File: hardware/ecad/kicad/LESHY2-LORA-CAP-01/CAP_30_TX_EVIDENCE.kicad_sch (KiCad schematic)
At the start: 0 parts

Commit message: complete H2.4.2 LoRa Cap root
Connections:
- no-connect marks 0 -> 4
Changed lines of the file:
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@@
 	(generator_version "10.0")
 	(paper "A4")
+	(hierarchical_label "CAP_3V3"
+		(shape bidirectional)
+		(at 20.32 20.32 0)
+		(effects (font (size 1.27 1.27)))
+	)
+	(wire
+		(pts (xy 20.32 20.32) (xy 25.40 20.32))
+		(stroke (width 0) (type default))
+	)
+	(no_connect (at 25.40 20.32)
+	)
+	(hierarchical_label "GND"
+		(shape bidirectional)
+		(at 20.32 25.40 0)
+		(effects (font (size 1.27 1.27)))
+	)
+	(wire
+		(pts (xy 20.32 25.40) (xy 25.40 25.40))
+		(stroke (width 0) (type default))
+	)
+	(no_connect (at 25.40 25.40)
+	)
+	(hierarchical_label "RF_FORWARD_LEVEL"
+		(shape bidirectional)
+		(at 190.50 20.32 180)
+		(effects (font (size 1.27 1.27)) (justify right))
+	)
+	(wire
+		(pts (xy 190.50 20.32) (xy 185.42 20.32))
+		(stroke (width 0) (type default))
+	)
+	(no_connect (at 185.42 20.32)
+	)
+	(hierarchical_label "EXT_TX_EVIDENCE_N"
+		(shape bidirectional)
+		(at 190.50 25.40 180)
+		(effects (font (size 1.27 1.27)) (justify right))
+	)
+	(wire
+		(pts (xy 190.50 25.40) (xy 185.42 25.40))
+		(stroke (width 0) (type default))
+	)
+	(no_connect (at 185.42 25.40)
+	)
 	(sheet_instances
 		(path "/"

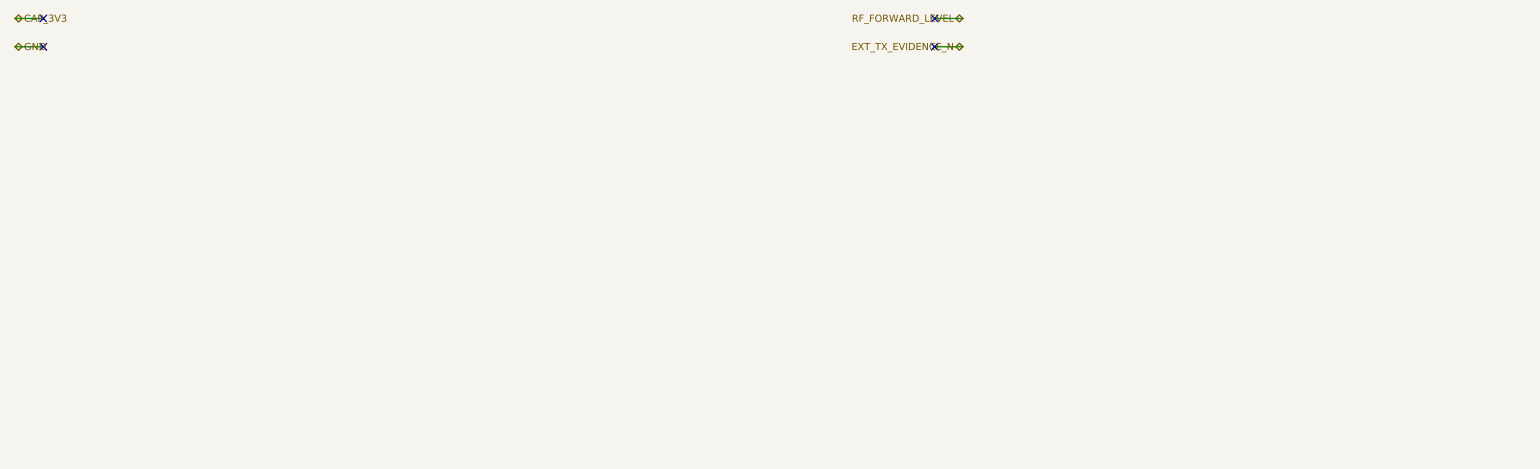
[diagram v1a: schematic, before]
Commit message: complete H2.4 LoRa Cap schematics
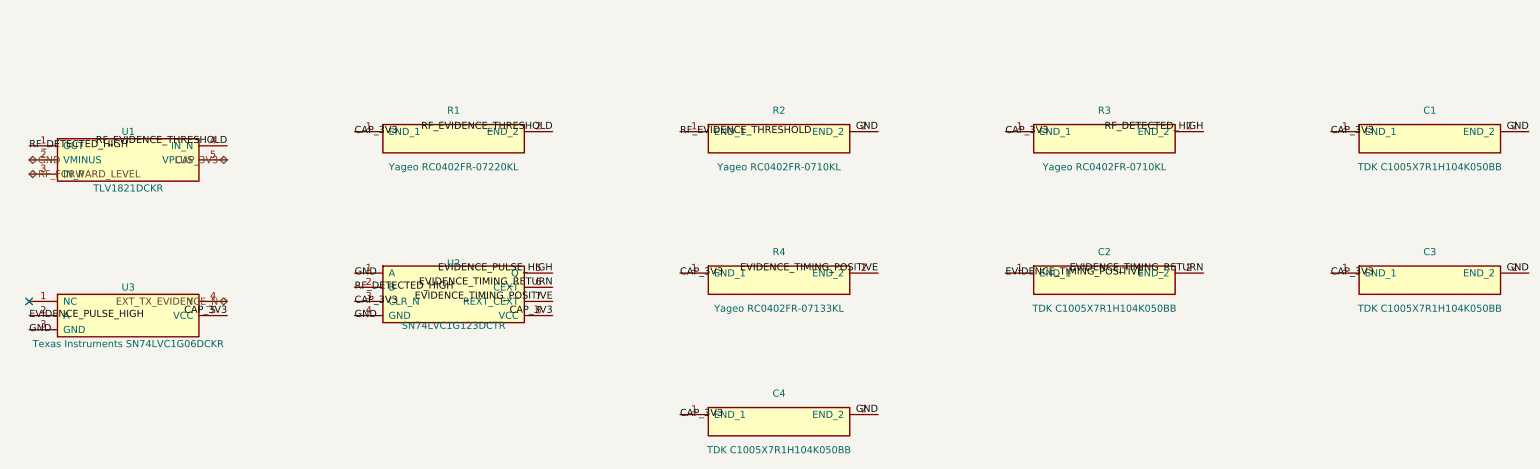
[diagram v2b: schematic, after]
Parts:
- added C1: TDK C1005X7R1H104K050BB, Capacitor_SMD:C_0402_1005Metric, symbol Leshy2:CAP30_EVIDENCE_COMPARATOR_BYPASS
- added C2: TDK C1005X7R1H104K050BB, Capacitor_SMD:C_0402_1005Metric, symbol Leshy2:CAP30_EVIDENCE_TIMING_CAPACITOR
- added C3: TDK C1005X7R1H104K050BB, Capacitor_SMD:C_0402_1005Metric, symbol Leshy2:CAP30_EVIDENCE_MONOSTABLE_BYPASS
- added C4: TDK C1005X7R1H104K050BB, Capacitor_SMD:C_0402_1005Metric, symbol Leshy2:CAP30_EVIDENCE_DRIVER_BYPASS
- added R1: Yageo RC0402FR-07220KL, Resistor_SMD:R_0402_1005Metric, symbol Leshy2:CAP30_EVIDENCE_THRESHOLD_TOP
- added R2: Yageo RC0402FR-0710KL, Resistor_SMD:R_0402_1005Metric, symbol Leshy2:CAP30_EVIDENCE_THRESHOLD_BOTTOM
- added R3: Yageo RC0402FR-0710KL, Resistor_SMD:R_0402_1005Metric, symbol Leshy2:CAP30_EVIDENCE_COMPARATOR_PULLUP
- added R4: Yageo RC0402FR-07133KL, Resistor_SMD:R_0402_1005Metric, symbol Leshy2:CAP30_EVIDENCE_TIMING_RESISTOR
- added U1: TLV1821DCKR, Package_TO_SOT_SMD:Texas_R-PDSO-G5_DCK-5, symbol Leshy2:CAP30_EVIDENCE_COMPARATOR
- added U2: SN74LVC1G123DCTR, Package_SO:SSOP-8_2.95x2.8mm_P0.65mm, symbol Leshy2:CAP30_EVIDENCE_MONOSTABLE
- added U3: Texas Instruments SN74LVC1G06DCKR, Package_TO_SOT_SMD:Texas_R-PDSO-G5_DCK-5, symbol Leshy2:CAP30_EVIDENCE_DRIVER
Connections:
- net CAP_3V3: now also C1.1 (END_1), C3.1 (END_1), C4.1 (END_1), R1.1 (END_1), R3.1 (END_1), R4.1 (END_1), U1.5 (VPLUS), U2.3 (CLR_N), U2.8 (VCC), U3.5 (VCC)
- net EXT_TX_EVIDENCE_N: now also U3.4 (Y)
- net GND: now also C1.2 (END_2), C3.2 (END_2), C4.2 (END_2), R2.2 (END_2), U1.2 (VMINUS), U2.1 (A), U2.4 (GND), U3.3 (GND)
- net RF_FORWARD_LEVEL: now also U1.3 (IN_P)
- new net EVIDENCE_PULSE_HIGH: U2.5 (Q), U3.2 (A)
- new net EVIDENCE_TIMING_POSITIVE: C2.1 (END_1), R4.2 (END_2), U2.7 (REXT_CEXT)
- new net EVIDENCE_TIMING_RETURN: C2.2 (END_2), U2.6 (CEXT)
- new net RF_DETECTED_HIGH: R3.2 (END_2), U1.1 (OUT), U2.2 (B)
- new net RF_EVIDENCE_THRESHOLD: R1.2 (END_2), R2.1 (END_1), U1.4 (IN_N)
- no-connect marks 4 -> 1
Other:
- title: (none) -> Leshy2 LoRa Cap — independent physical-TX evidence pulse
